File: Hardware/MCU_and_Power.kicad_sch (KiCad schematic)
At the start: 3 parts, among them J1 Conn_01x20_Socket, J2 Conn_01x20_Socket

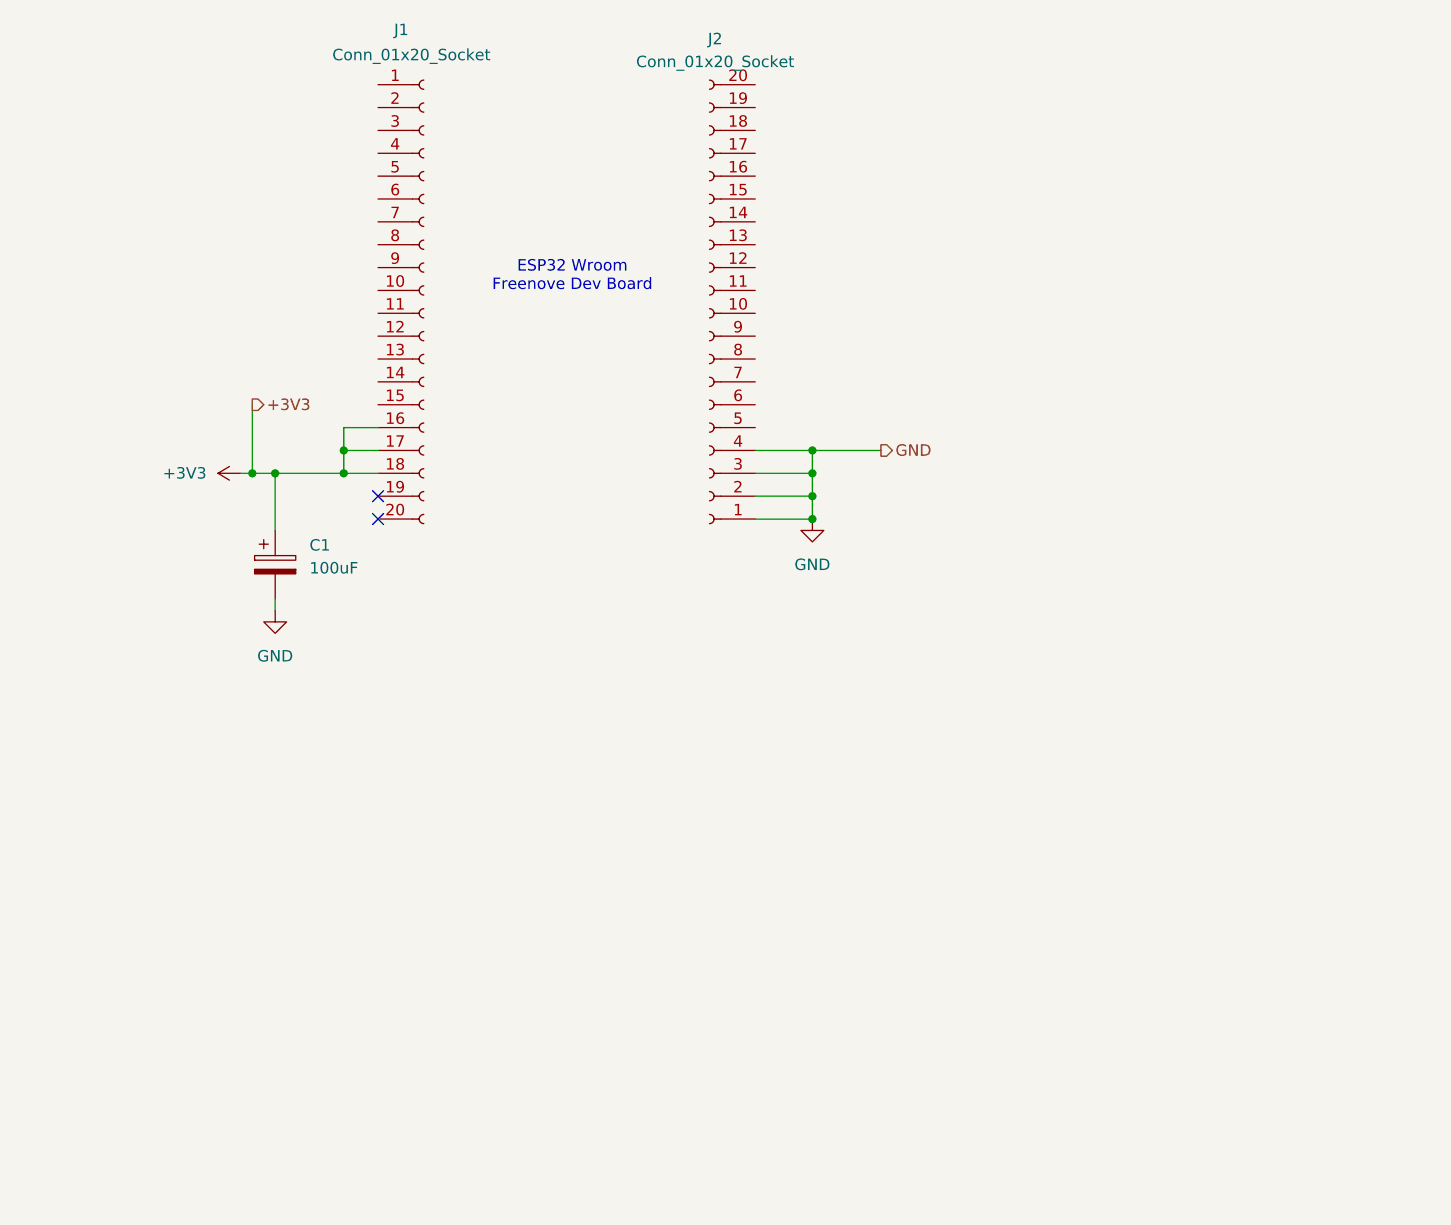
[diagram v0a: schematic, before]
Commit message: Major Updates to Schematic
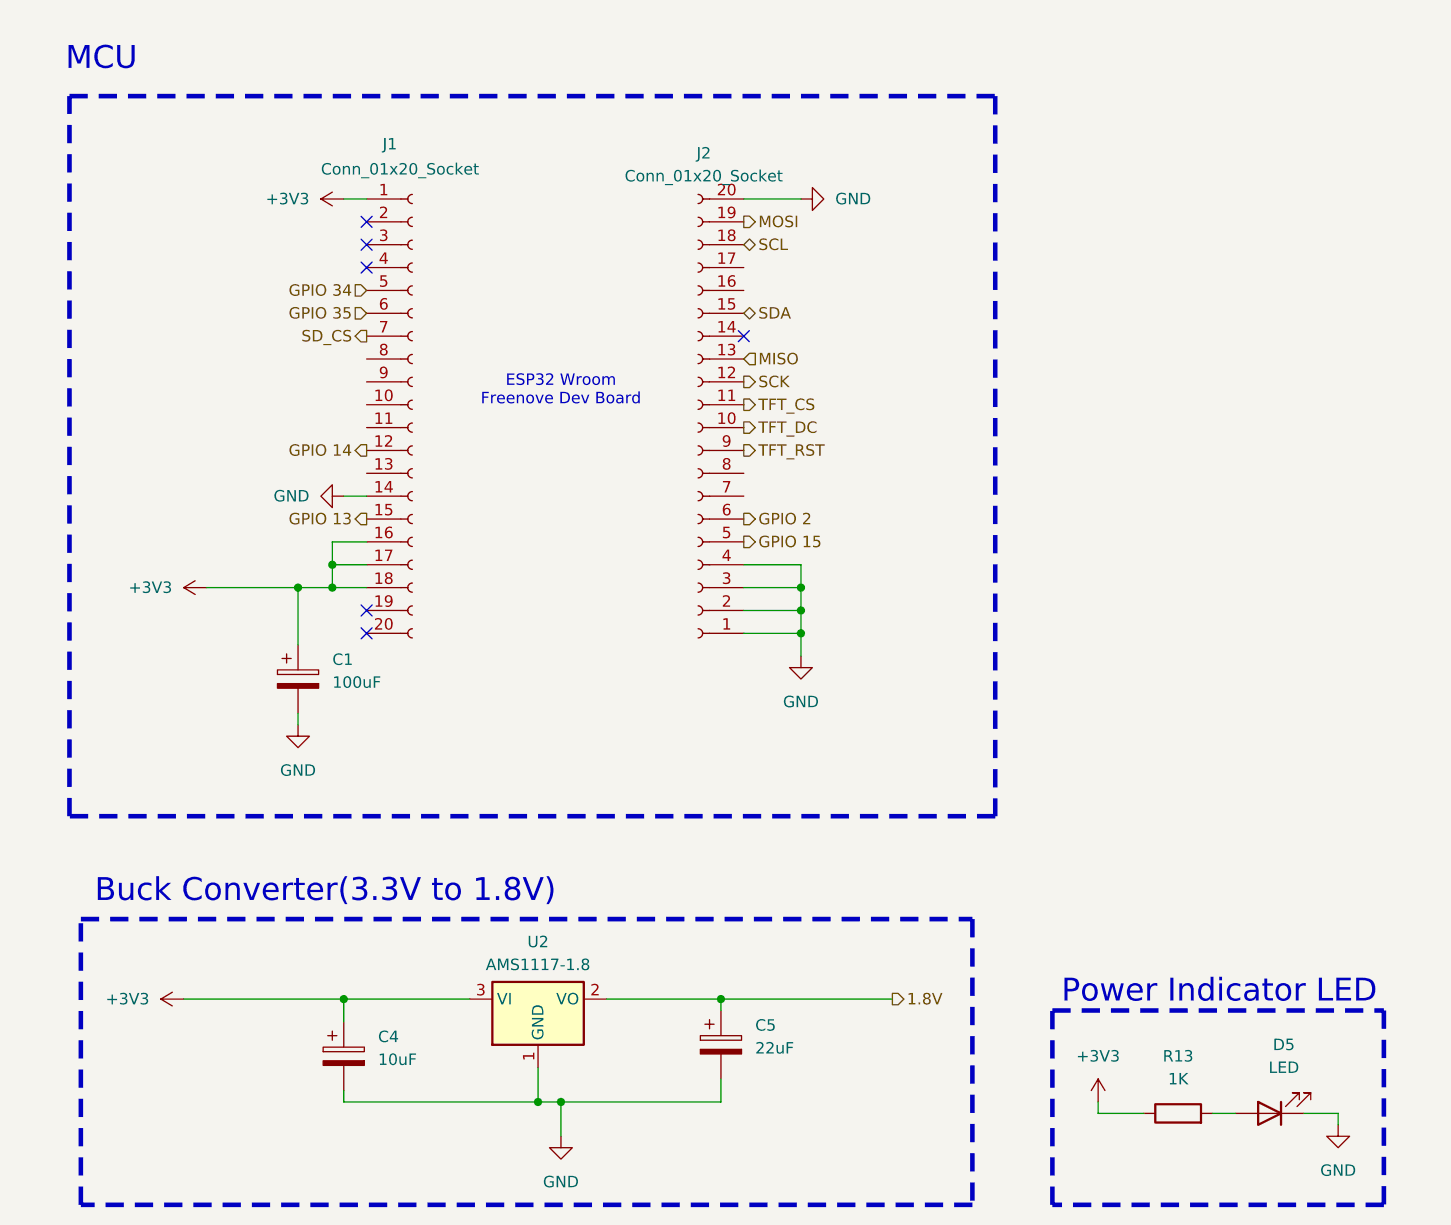
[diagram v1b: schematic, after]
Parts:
- added C4: 10uF, symbol Device:C_Polarized
- added C5: 22uF, symbol Device:C_Polarized
- added D5: LED, symbol Device:LED
- added R13: 1K, symbol Device:R
- added U2: AMS1117-1.8, Package_TO_SOT_SMD:SOT-223-3_TabPin2, symbol Regulator_Linear:AMS1117-1.8
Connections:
- net +3V3: now also J1.1 (Pin_1), C4.1, R13.1, U2.3 (VI)
- net GND: now also J1.14 (Pin_14), J2.20 (Pin_20), C4.2, C5.2, D5.1 (K), U2.1 (GND)
- net TFT_DC: now reaches J2.10 (Pin_10)
- net TFT_CS: now reaches J2.11 (Pin_11)
- net SCK: now reaches J2.12 (Pin_12)
- net MISO: now reaches J2.13 (Pin_13)
- net SDA: now reaches J2.15 (Pin_15)
- net SCL: now reaches J2.18 (Pin_18)
- net MOSI: now reaches J2.19 (Pin_19)
- net GPIO 15: now reaches J2.5 (Pin_5)
- net GPIO 2: now reaches J2.6 (Pin_6)
- net TFT_RST: now reaches J2.9 (Pin_9)
- net GPIO 14: now reaches J1.12 (Pin_12)
- net GPIO 13: now reaches J1.15 (Pin_15)
- net GPIO 34: now reaches J1.5 (Pin_5)
- net GPIO 35: now reaches J1.6 (Pin_6)
- net SD_CS: now reaches J1.7 (Pin_7)
- new net: D5.2 (A), R13.2
- new net 1.8V: C5.1, U2.2 (VO)
- no-connect marks 2 -> 6
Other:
- note added: "Buck Converter(3.3V to 1.8V)"
- note added: "MCU"
- note added: "Power Indicator LED"
- moved on the sheet: C1, J1, J2
